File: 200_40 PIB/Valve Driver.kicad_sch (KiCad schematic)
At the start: 6 parts, among them J12 532610671, Q5 NMOS, U12 DRV8220DRL, U13 DRV8220DRL

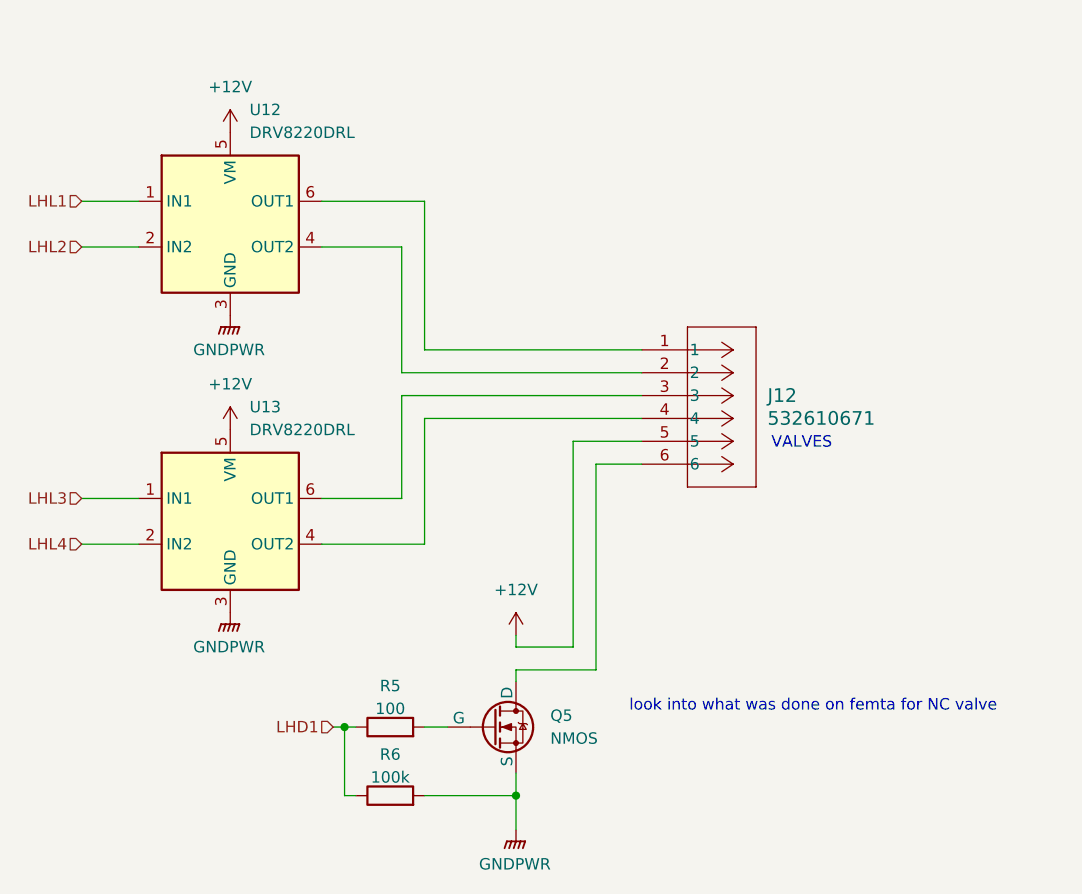
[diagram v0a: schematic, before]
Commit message: .nhoj
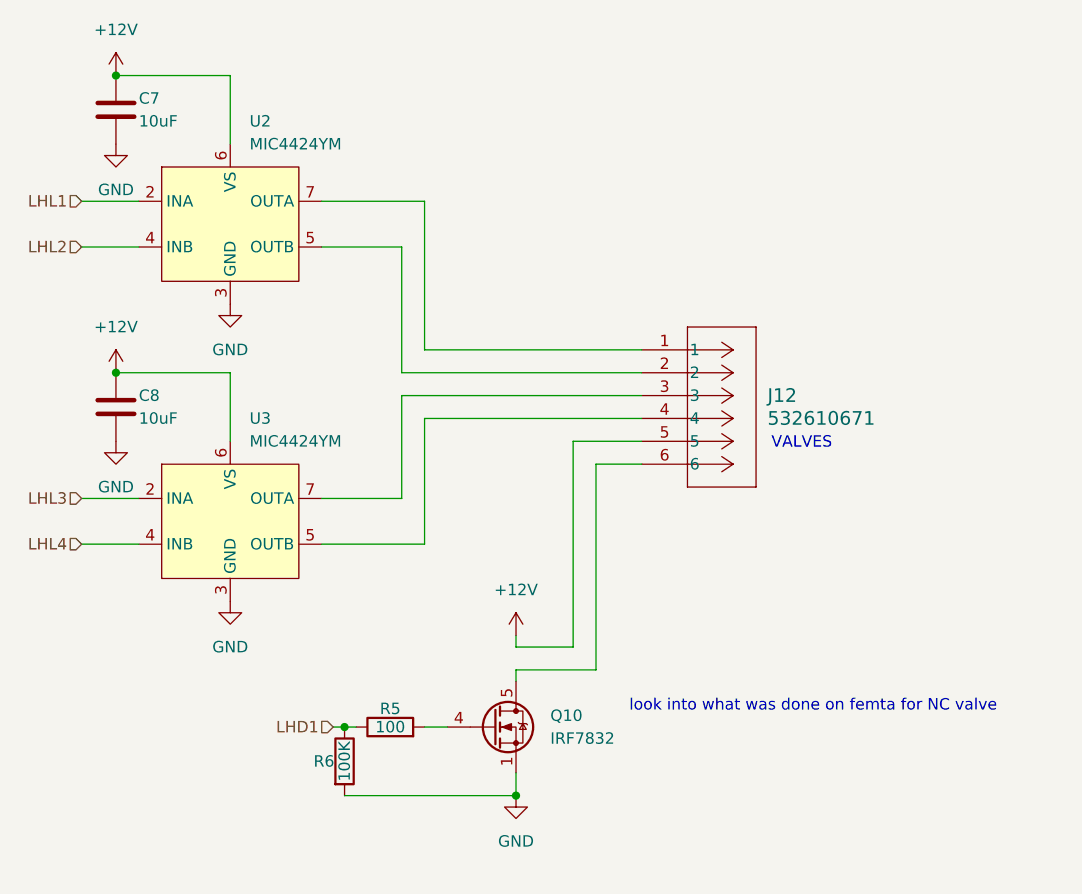
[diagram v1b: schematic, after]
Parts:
- removed Q5: NMOS, symbol Simulation_SPICE:NMOS
- removed U12, U13: DRV8220DRL, Package_TO_SOT_SMD:SOT-563, symbol Driver_Motor:DRV8220DRL
- added C7, C8: 10uF, Capacitor_SMD:C_0805_2012Metric, symbol Device:C
- added Q10: IRF7832, Package_SO:SOIC-8_3.9x4.9mm_P1.27mm, symbol Transistor_FET:IRF7403
- added U2, U3: MIC4424YM, Package_SO:SOIC-8_3.9x4.9mm_P1.27mm, symbol MIC4424YM:MIC4424YM
- R6: value 100k -> 100K
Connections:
- net +12V: now also C7.1, C8.1, U2.6 (VS), U3.6 (VS)
- net LHL1: now also U2.2 (INA)
- net LHL2: now also U2.4 (INB)
- net LHL3: now also U3.2 (INA)
- net LHL4: now also U3.4 (INB)
- net at J12.6: now also Q10.5 (D), Q10.6 (D), Q10.7 (D), Q10.8 (D)
- net at R5.2: now also Q10.4 (G)
- net at J12.1: now also U2.7 (OUTA)
- net at J12.2: now also U2.5 (OUTB)
- net at J12.3: now also U3.7 (OUTA)
- net at J12.4: now also U3.5 (OUTB)
- net GNDPWR renamed GND
- net GND: now also C7.2, C8.2, Q10.1 (S), Q10.2 (S), Q10.3 (S), U2.3 (GND), U3.3 (GND)
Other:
- moved on the sheet: R6
